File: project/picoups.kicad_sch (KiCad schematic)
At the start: 44 parts, among them J1 Conn_02x20_Odd_Even, J2 BATT, J3 VIN, J4 5V, Q1 Q_PMOS_GSD, U1 LT3652EMSE, U2 INA3221, U3 TPS61235P

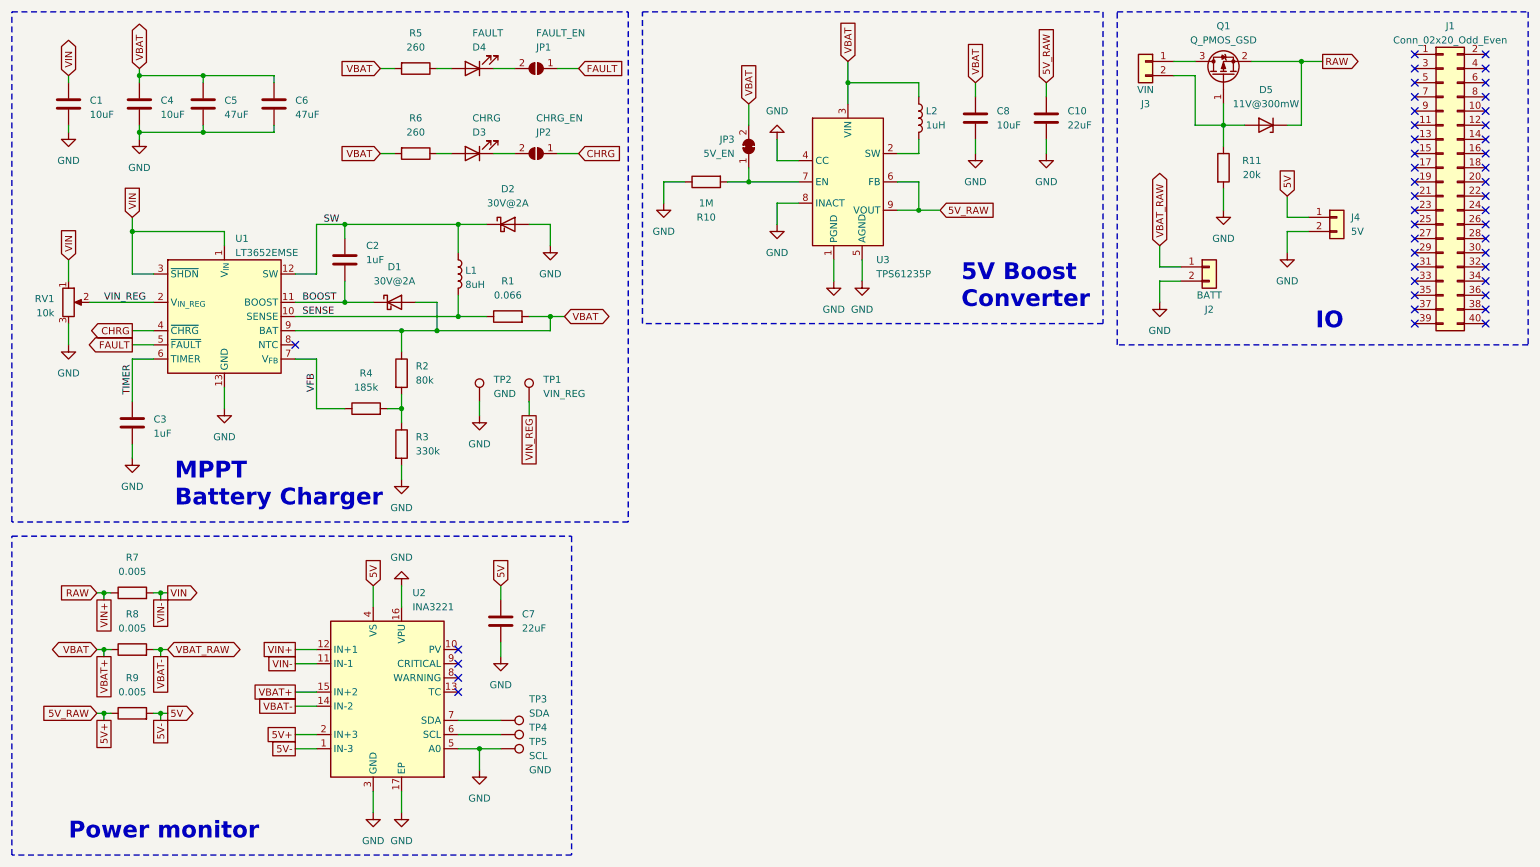
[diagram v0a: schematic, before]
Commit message: Added components
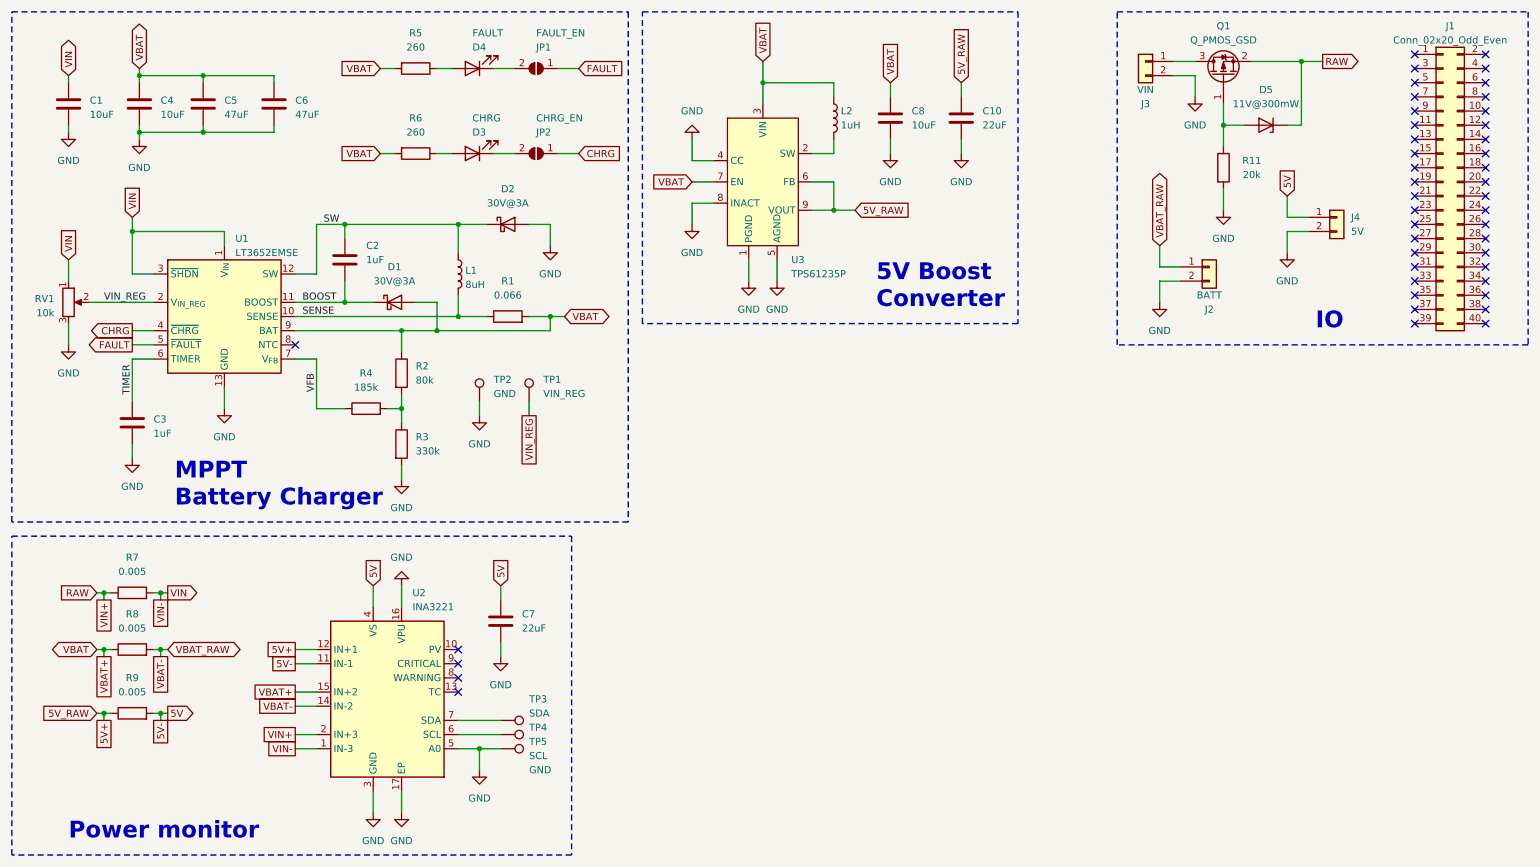
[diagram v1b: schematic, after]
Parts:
- removed JP3: 5V_EN, Jumper:SolderJumper-2_P1.3mm_Bridged_RoundedPad1.0x1.5mm, symbol Jumper:SolderJumper_2_Bridged
- removed R10: 1M, Resistor_SMD:R_0805_2012Metric, symbol Device:R
- D1, D2: value 30V@2A -> 30V@3A; footprint Diode_SMD:D_MicroSMP_AK -> Diode_SMD:D_SOD-123F
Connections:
- net 5V: now also U2.11 (IN-1); no longer U2.1 (IN-3)
- net 5V+: now also U2.12 (IN+1); no longer U2.2 (IN+3)
- net GND: now also J3.2 (Pin_2)
- net RAW: now also U2.2 (IN+3); no longer U2.12 (IN+1)
- net VBAT: now also U3.7 (EN)
- net VIN: now also U2.1 (IN-3); no longer U2.11 (IN-1)
- net at D5.2 (A), Q1.1 (G), R11.1: no longer J3.2 (Pin_2)
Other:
- moved on the sheet: C10, C8, L2, U3
